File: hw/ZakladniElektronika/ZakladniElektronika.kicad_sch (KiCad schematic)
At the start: 0 parts

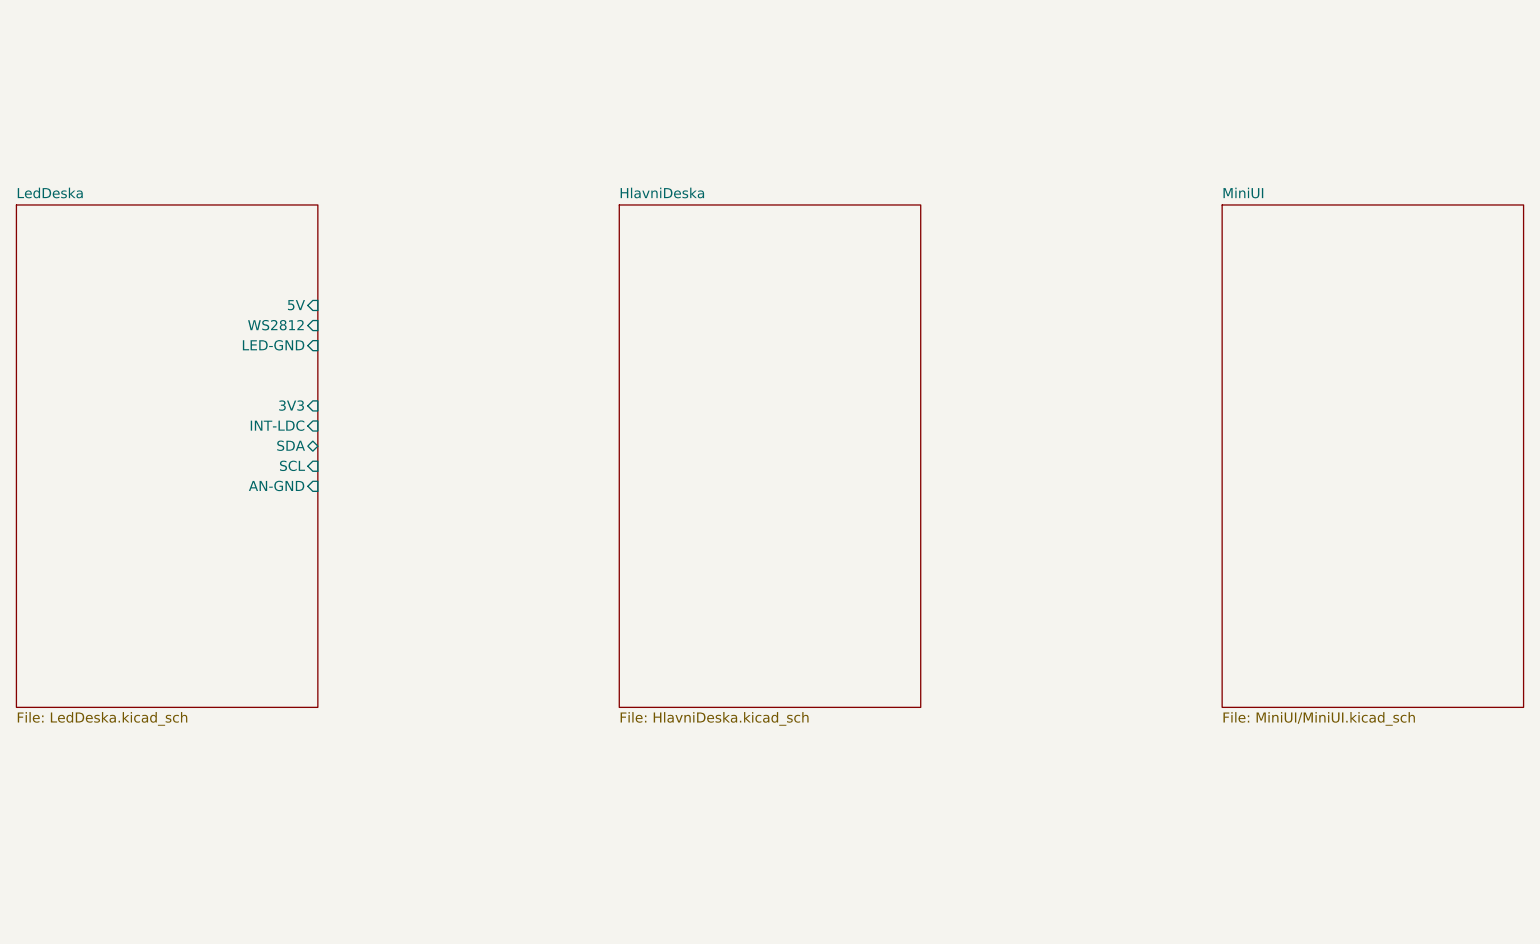
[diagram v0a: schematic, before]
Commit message: Nastin schematu
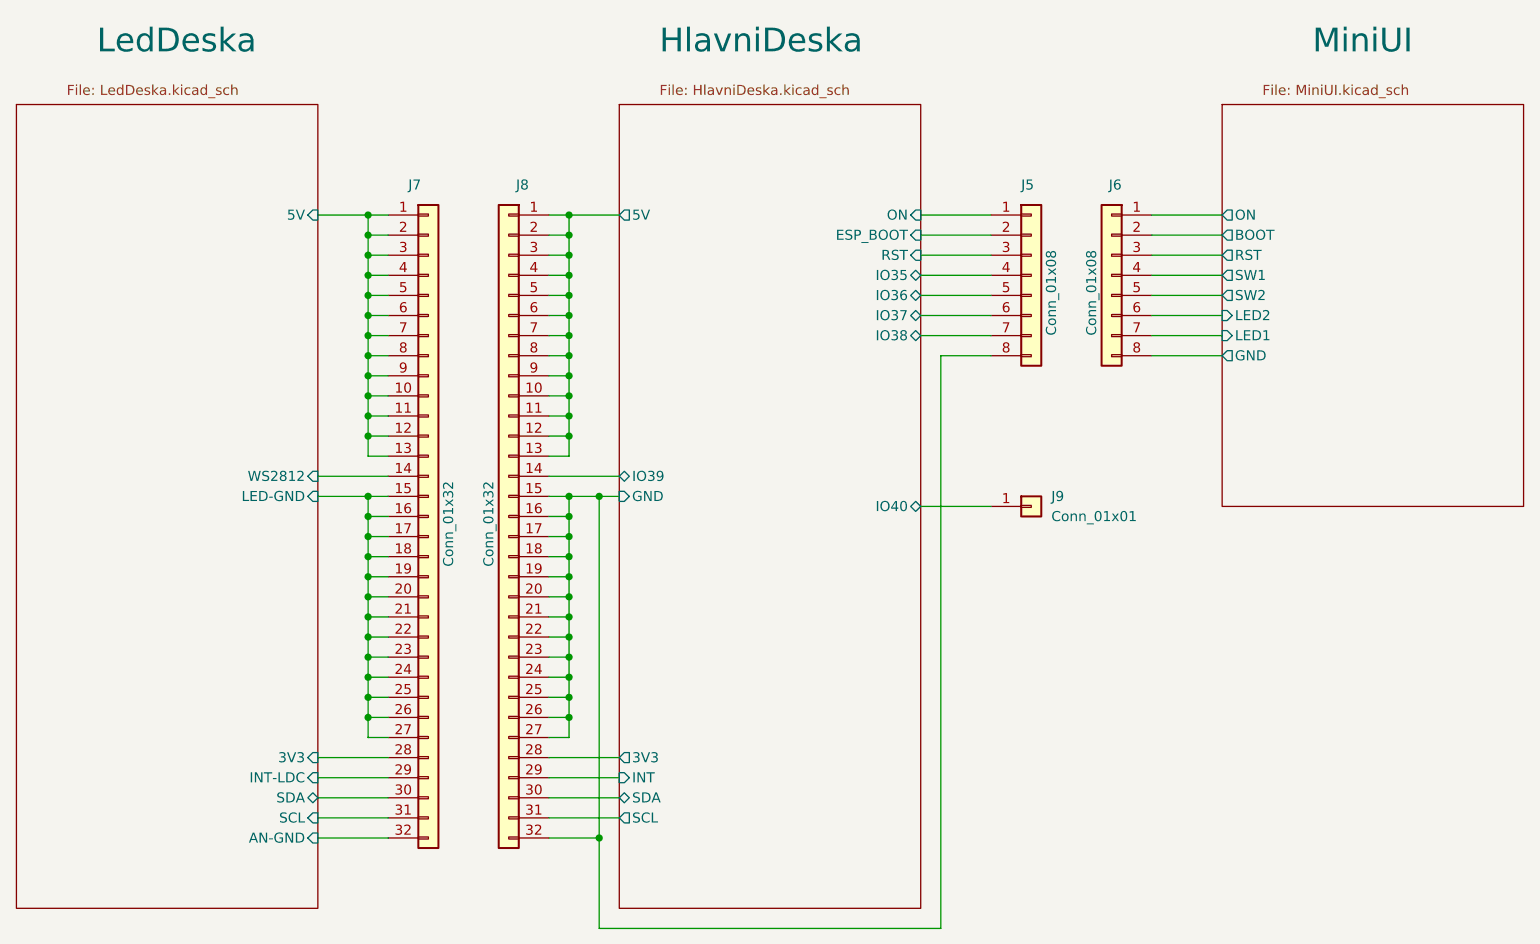
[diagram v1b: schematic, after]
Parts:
- added J5, J6: Conn_01x08, Connector_JST:JST_EH_B8B-EH-A_1x08_P2.50mm_Vertical, symbol Connector_Generic:Conn_01x08
- added J7, J8: Conn_01x32, Connector_FFC-FPC:TE_3-1734839-2_1x32-1MP_P0.5mm_Horizontal, symbol Connector_Generic:Conn_01x32
- added J9: Conn_01x01, Connector_PinHeader_2.54mm:PinHeader_1x01_P2.54mm_Vertical, symbol Connector_Generic:Conn_01x01
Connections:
- net LedDeska/3V3: now also J7.28 (Pin_28)
- net LedDeska/5V: now also J7.1 (Pin_1), J7.10 (Pin_10), J7.11 (Pin_11), J7.12 (Pin_12), J7.13 (Pin_13), J7.2 (Pin_2), J7.3 (Pin_3), J7.4 (Pin_4), J7.5 (Pin_5), J7.6 (Pin_6), J7.7 (Pin_7), J7.8 (Pin_8), J7.9 (Pin_9)
- net LedDeska/AN-GND: now also J7.32 (Pin_32)
- net LedDeska/INT-LDC: now also J7.29 (Pin_29)
- net LedDeska/LED-GND: now also J7.15 (Pin_15), J7.16 (Pin_16), J7.17 (Pin_17), J7.18 (Pin_18), J7.19 (Pin_19), J7.20 (Pin_20), J7.21 (Pin_21), J7.22 (Pin_22), J7.23 (Pin_23), J7.24 (Pin_24), J7.25 (Pin_25), J7.26 (Pin_26), J7.27 (Pin_27)
- net LedDeska/SCL: now also J7.31 (Pin_31)
- net LedDeska/SDA: now also J7.30 (Pin_30)
- net LedDeska/WS2812: now also J7.14 (Pin_14)
- new net HlavniDeska/3V3: J8.28 (Pin_28)
- new net HlavniDeska/5V: J8.1 (Pin_1), J8.10 (Pin_10), J8.11 (Pin_11), J8.12 (Pin_12), J8.13 (Pin_13), J8.2 (Pin_2), J8.3 (Pin_3), J8.4 (Pin_4), J8.5 (Pin_5), J8.6 (Pin_6), J8.7 (Pin_7), J8.8 (Pin_8), J8.9 (Pin_9)
- new net HlavniDeska/ESP_BOOT: J5.2 (Pin_2)
- new net HlavniDeska/GND: J5.8 (Pin_8), J8.15 (Pin_15), J8.16 (Pin_16), J8.17 (Pin_17), J8.18 (Pin_18), J8.19 (Pin_19), J8.20 (Pin_20), J8.21 (Pin_21), J8.22 (Pin_22), J8.23 (Pin_23), J8.24 (Pin_24), J8.25 (Pin_25), J8.26 (Pin_26), J8.27 (Pin_27), J8.32 (Pin_32)
- new net HlavniDeska/INT: J8.29 (Pin_29)
- new net HlavniDeska/IO35: J5.4 (Pin_4)
- new net HlavniDeska/IO36: J5.5 (Pin_5)
- new net HlavniDeska/IO37: J5.6 (Pin_6)
- new net HlavniDeska/IO38: J5.7 (Pin_7)
- new net HlavniDeska/IO39: J8.14 (Pin_14)
- new net HlavniDeska/IO40: J9.1 (Pin_1)
- new net HlavniDeska/ON: J5.1 (Pin_1)
- new net HlavniDeska/RST: J5.3 (Pin_3)
- new net HlavniDeska/SCL: J8.31 (Pin_31)
- new net HlavniDeska/SDA: J8.30 (Pin_30)
- new net MiniUI/BOOT: J6.2 (Pin_2)
- new net MiniUI/GND: J6.8 (Pin_8)
- new net MiniUI/LED1: J6.7 (Pin_7)
- new net MiniUI/LED2: J6.6 (Pin_6)
- new net MiniUI/ON: J6.1 (Pin_1)
- new net MiniUI/RST: J6.3 (Pin_3)
- new net MiniUI/SW1: J6.4 (Pin_4)
- new net MiniUI/SW2: J6.5 (Pin_5)
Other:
- sheet HlavniDeska ports: added 3V3, 5V, ESP_BOOT, GND, INT, IO35, IO36, IO37, IO38, IO39, IO40, ON, RST, SCL, SDA; removed none
- sheet MiniUI: file MiniUI/MiniUI.kicad_sch -> MiniUI.kicad_sch
- sheet MiniUI ports: added BOOT, GND, LED1, LED2, ON, RST, SW1, SW2; removed none
